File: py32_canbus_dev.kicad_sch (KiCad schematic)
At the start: 42 parts, among them J2 Conn_01x18, J3 Conn_01x18, J4 CAN1, J5 USB_B_Micro, SW2 Reset, U1 uA7805, U2 PY32F030K1xT, U3 MCP2518FD-E/QBB, U4 MCP2562FD-E/MF, U5 FT230XQ, Y1 24MHz, Y2 40MHz

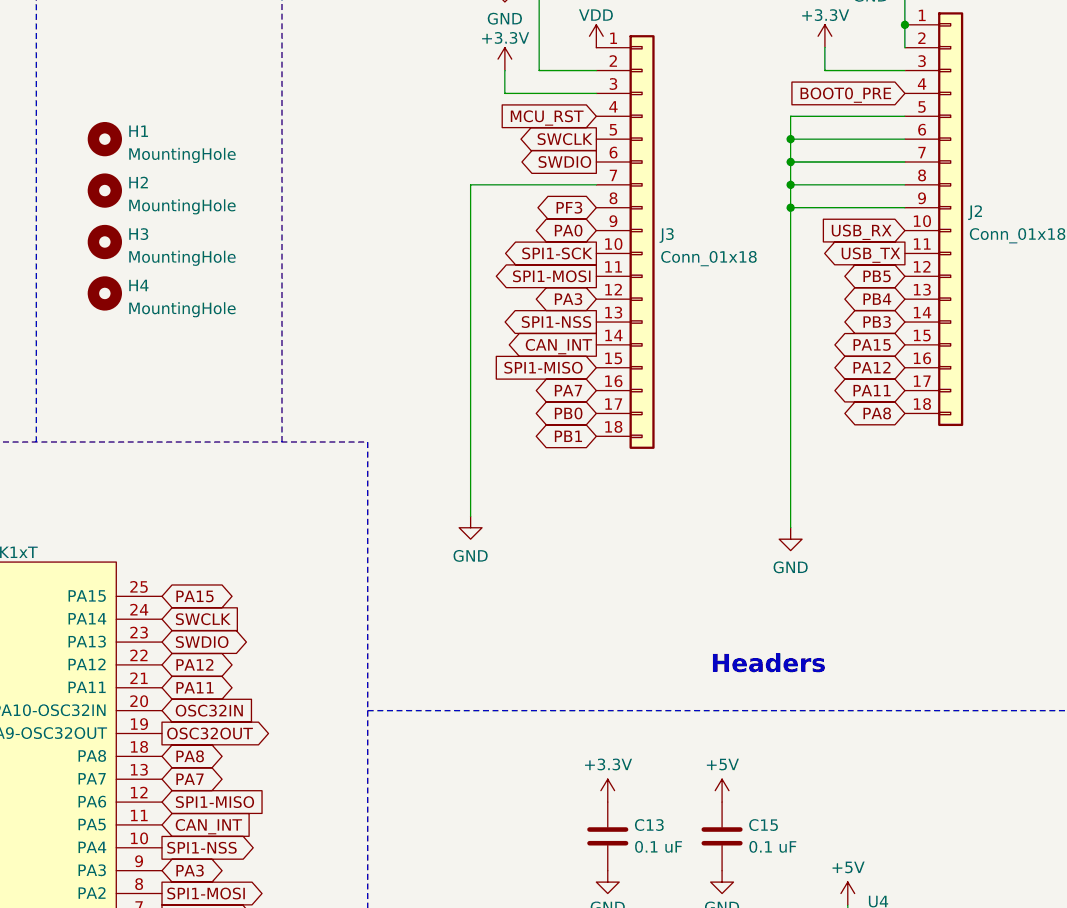
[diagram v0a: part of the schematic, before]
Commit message: Completed schematic and pcb check
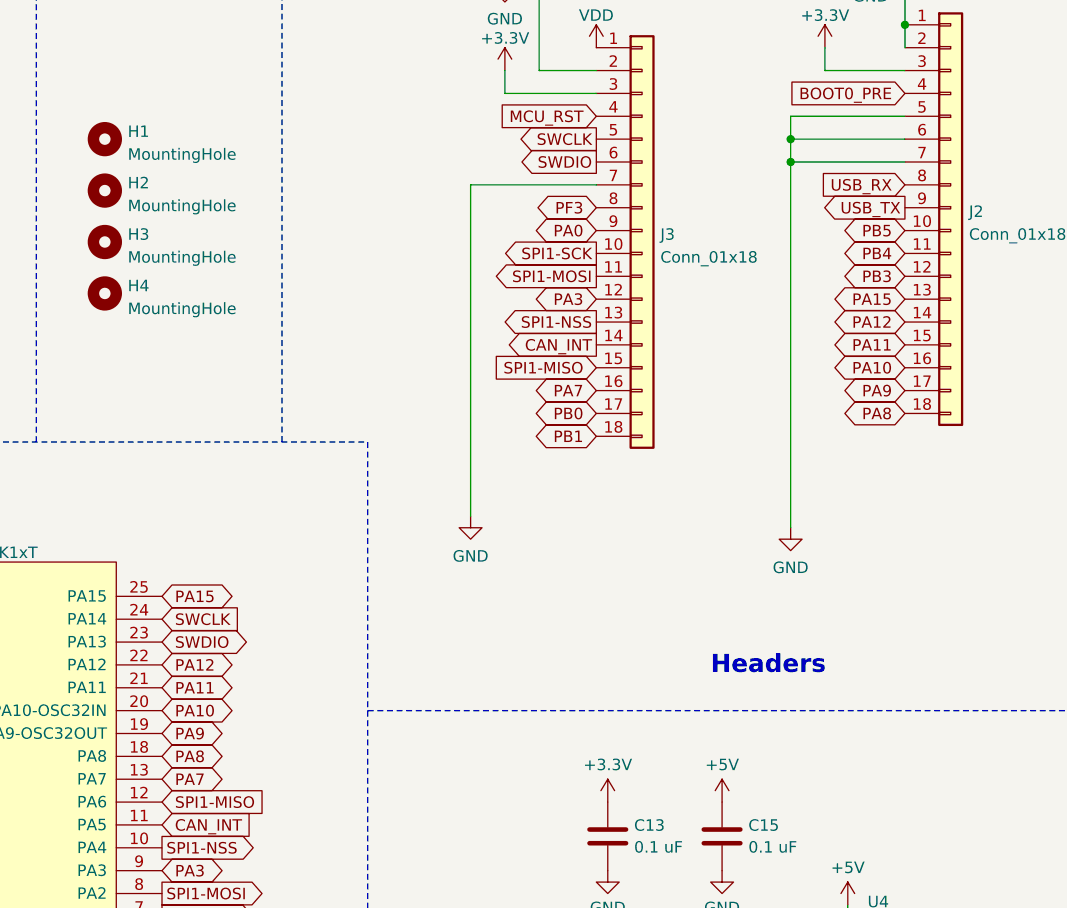
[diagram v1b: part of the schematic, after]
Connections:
- net GND: no longer J2.8 (Pin_8), J2.9 (Pin_9)
- net PA11: now also J2.15 (Pin_15); no longer J2.17 (Pin_17)
- net PA12: now also J2.14 (Pin_14); no longer J2.16 (Pin_16)
- net PA15: now also J2.13 (Pin_13); no longer J2.15 (Pin_15)
- net PB3: now also J2.12 (Pin_12); no longer J2.14 (Pin_14)
- net PB4: now also J2.11 (Pin_11); no longer J2.13 (Pin_13)
- net PB5: now also J2.10 (Pin_10); no longer J2.12 (Pin_12)
- net USB_RX: now also J2.8 (Pin_8); no longer J2.10 (Pin_10)
- net USB_TX: now also J2.9 (Pin_9); no longer J2.11 (Pin_11)
- net OSC32IN renamed PA10
- net PA10: now also J2.16 (Pin_16)
- net OSC32OUT renamed PA9
- net PA9: now also J2.17 (Pin_17)
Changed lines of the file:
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@@
 	)
 	(junction
-		(at 232.41 44.45)
-		(diameter 0)
-		(color 0 0 0 0)
-	)
-	(junction
 		(at 130.81 34.29)
 		(diameter 0)
@@
 	)
 	(junction
-		(at 232.41 46.99)
-		(diameter 0)
-		(color 0 0 0 0)
-	)
-	(junction
 		(at 238.76 147.32)
 		(diameter 0)
@@
 	(wire
 		(pts
-			(xy 232.41 46.99) (xy 232.41 82.55)
-		)
-		(stroke
-			(width 0)
-			(type default)
-		)
-	)
-	(wire
-		(pts
 			(xy 52.07 135.89) (xy 52.07 139.7)
 		)
@@
 	(wire
 		(pts
-			(xy 232.41 41.91) (xy 232.41 44.45)
+			(xy 232.41 41.91) (xy 232.41 82.55)
 		)
 		(stroke
@@
 	(wire
 		(pts
-			(xy 232.41 46.99) (xy 245.11 46.99)
-		)
-		(stroke
-			(width 0)
-			(type default)
-		)
-	)
-	(wire
-		(pts
 			(xy 139.7 175.26) (xy 139.7 177.8)
 		)
@@
 	(wire
 		(pts
-			(xy 232.41 44.45) (xy 232.41 46.99)
-		)
-		(stroke
-			(width 0)
-			(type default)
-		)
-	)
-	(wire
-		(pts
-			(xy 232.41 44.45) (xy 245.11 44.45)
-		)
-		(stroke
-			(width 0)
-			(type default)
-		)
-	)
-	(wire
-		(pts
 			(xy 27.94 59.69) (xy 27.94 49.53)
 		)
@@
 	(global_label "PA15"
 		(shape bidirectional)
-		(at 245.11 62.23 180)
+		(at 245.11 57.15 180)
+		(fields_autoplaced yes)
+		(effects
+			(font
+				(size 1.27 1.27)
+			)
+			(justify right)
+		)
+		(property "Intersheetrefs" "${INTERSHEET_REFS}"
+			(at 237.9193 57.2294 0)
+			(effects
+				(font
+					(size 1.27 1.27)
+				)
+				(justify right)
+				(hide yes)
+			)
+		)
+	)
+	(global_label "PA10"
+		(shape bidirectional)
+		(at 245.11 64.77 180)
 		(fields_autoplaced yes)
 		(effects
@@
 		)
 		(property "Intersheetrefs" "${INTERSHEET_REFS}"
-			(at 237.9193 62.3094 0)
+			(at 236.2359 64.77 0)
 			(effects
 				(font
@@
 		)
 	)
-	(global_label "OSC32OUT"
-		(shape output)
+	(global_label "PA9"
+		(shape bidirectional)
 		(at 162.56 105.41 0)
 		(fields_autoplaced yes)
@@
 		)
 		(property "Intersheetrefs" "${INTERSHEET_REFS}"
-			(at 174.8307 105.4894 0)
+			(at 170.2246 105.41 0)
 			(effects
 				(font
@@
 		)
 	)
-	(global_label "OSC32IN"
-		(shape input)
+	(global_label "PA10"
+		(shape bidirectional)
 		(at 162.56 102.87 0)
 		(fields_autoplaced yes)
@@
 		)
 		(property "Intersheetrefs" "${INTERSHEET_REFS}"
-			(at 173.1374 102.9494 0)
+			(at 171.4341 102.87 0)
 			(effects
 				(font
@@
 		)
 	)
+	(global_label "PA9"
+		(shape bidirectional)
+		(at 245.11 67.31 180)
+		(fields_autoplaced yes)
+		(effects
+			(font
+				(size 1.27 1.27)
+			)
+			(justify right)
+		)
+		(property "Intersheetrefs" "${INTERSHEET_REFS}"
+			(at 237.4454 67.31 0)
+			(effects
+				(font
+					(size 1.27 1.27)
+				)
+				(justify right)
+				(hide yes)
+			)
+		)
+	)
 	(global_label "SPI1-NSS"
 		(shape input)
@@
 	(global_label "PB4"
 		(shape bidirectional)
-		(at 245.11 57.15 180)
+		(at 245.11 52.07 180)
 		(fields_autoplaced yes)
 		(effects
@@
 		)
 		(property "Intersheetrefs" "${INTERSHEET_REFS}"
-			(at 238.9474 57.0706 0)
+			(at 238.9474 51.9906 0)
 			(effects
 				(font
@@
 	(global_label "PB3"
 		(shape bidirectional)
-		(at 245.11 59.69 180)
+		(at 245.11 54.61 180)
 		(fields_autoplaced yes)
 		(effects
@@
 		)
 		(property "Intersheetrefs" "${INTERSHEET_REFS}"
-			(at 238.9474 59.6106 0)
+			(at 238.9474 54.5306 0)
 			(effects
 				(font
@@
 	(global_label "USB_RX"
 		(shape input)
-		(at 245.11 49.53 180)
+		(at 245.11 44.45 180)
 		(fields_autoplaced yes)
 		(effects
@@
 		)
 		(property "Intersheetrefs" "${INTERSHEET_REFS}"
-			(at 234.8677 49.53 0)
+			(at 234.8677 44.45 0)
 			(effects
 				(font
@@
 	(global_label "USB_TX"
 		(shape output)
-		(at 245.11 52.07 180)
+		(at 245.11 46.99 180)
 		(fields_autoplaced yes)
 		(effects
@@
 		)
 		(property "Intersheetrefs" "${INTERSHEET_REFS}"
-			(at 235.1701 52.07 0)
+			(at 235.1701 46.99 0)
 			(effects
 				(font
@@
 	(global_label "PB5"
 		(shape bidirectional)
-		(at 245.11 54.61 180)
+		(at 245.11 49.53 180)
 		(fields_autoplaced yes)
 		(effects
@@
 		)
 		(property "Intersheetrefs" "${INTERSHEET_REFS}"
-			(at 238.9474 54.5306 0)
+			(at 238.9474 49.4506 0)
 			(effects
 				(font
@@
 	(global_label "PA12"
 		(shape bidirectional)
-		(at 245.11 64.77 180)
+		(at 245.11 59.69 180)
 		(fields_autoplaced yes)
 		(effects
@@
 		)
 		(property "Intersheetrefs" "${INTERSHEET_REFS}"
-			(at 237.9193 64.6906 0)
+			(at 237.9193 59.6106 0)
 			(effects
 				(font
@@
 	(global_label "PA11"
 		(shape bidirectional)
-		(at 245.11 67.31 180)
+		(at 245.11 62.23 180)
 		(fields_autoplaced yes)
 		(effects
@@
 		)
 		(property "Intersheetrefs" "${INTERSHEET_REFS}"
-			(at 237.9193 67.2306 0)
+			(at 237.9193 62.1506 0)
 			(effects
 				(font
@@
 			(at 238.76 135.89 0)
 			(effects
-				(font
-					(size 1.27 1.27)
-				)
-				(hide yes)
-			)
-		)
-		(property "Field5" ""
-			(at 238.76 135.89 0)
-			(effects
